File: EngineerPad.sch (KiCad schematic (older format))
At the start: 64 parts, among them J1 AVR ISP, J2 USB_A, SW1 SW_Push, SW10 SW_Push, SW11 SW_Push, SW12 SW_Push, SW13 SW_Push, SW14 SW_Push, SW15 SW_Push, SW16 SW_Push, SW17 SW_Push, SW18 SW_Push, SW19 SW_Push, SW2 SW_Push, SW20 SW_Push, SW21 SW_Push, SW22 SW_Push, SW23 SW_Push, SW3 SW_Push, SW4 SW_Push, SW5 SW_Push, SW6 SW_Push, SW7 SW_Push, SW8 SW_Push, SW9 SW_Push, U1 ATmega328P-PU, Y1 16MHz

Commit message: socket and low profile
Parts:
- SW21, SW22, SW23: footprint Button_Switch_Keyboard:SW_Cherry_MX_1.00u_PCB -> JSA:SW_PG1350
- U1: footprint Package_DIP:DIP-28_W7.62mm -> Package_DIP:DIP-28_W7.62mm_Socket
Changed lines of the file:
@@
 F 0 "U1" H 1206 3746 50  0000 R CNN
 F 1 "ATmega328P-PU" H 1206 3655 50  0000 R CNN
-F 2 "Package_DIP:DIP-28_W7.62mm" H 1850 3700 50  0001 C CIN
+F 2 "Package_DIP:DIP-28_W7.62mm_Socket" H 1850 3700 50  0001 C CIN
 F 3 "http://ww1.microchip.com/downloads/en/DeviceDoc/ATmega328_P%20AVR%20MCU%20with%20picoPower%20Technology%20Data%20Sheet%2040001984A.pdf" H 1850 3700 50  0001 C CNN
 	1    1850 3700
@@
 F 0 "SW23" H 10550 4685 50  0000 C CNN
 F 1 "SW_Push" H 10550 4594 50  0000 C CNN
-F 2 "Button_Switch_Keyboard:SW_Cherry_MX_1.00u_PCB" H 10550 4600 50  0001 C CNN
+F 2 "JSA:SW_PG1350" H 10550 4600 50  0001 C CNN
 F 3 "~" H 10550 4600 50  0001 C CNN
 	1    10550 4400
@@
 F 0 "SW22" H 10050 4685 50  0000 C CNN
 F 1 "SW_Push" H 10050 4594 50  0000 C CNN
-F 2 "Button_Switch_Keyboard:SW_Cherry_MX_1.00u_PCB" H 10050 4600 50  0001 C CNN
+F 2 "JSA:SW_PG1350" H 10050 4600 50  0001 C CNN
 F 3 "~" H 10050 4600 50  0001 C CNN
 	1    10050 4400
@@
 F 0 "SW21" H 9550 4685 50  0000 C CNN
 F 1 "SW_Push" H 9550 4594 50  0000 C CNN
-F 2 "Button_Switch_Keyboard:SW_Cherry_MX_1.00u_PCB" H 9550 4600 50  0001 C CNN
+F 2 "JSA:SW_PG1350" H 9550 4600 50  0001 C CNN
 F 3 "~" H 9550 4600 50  0001 C CNN
 	1    9550 4400

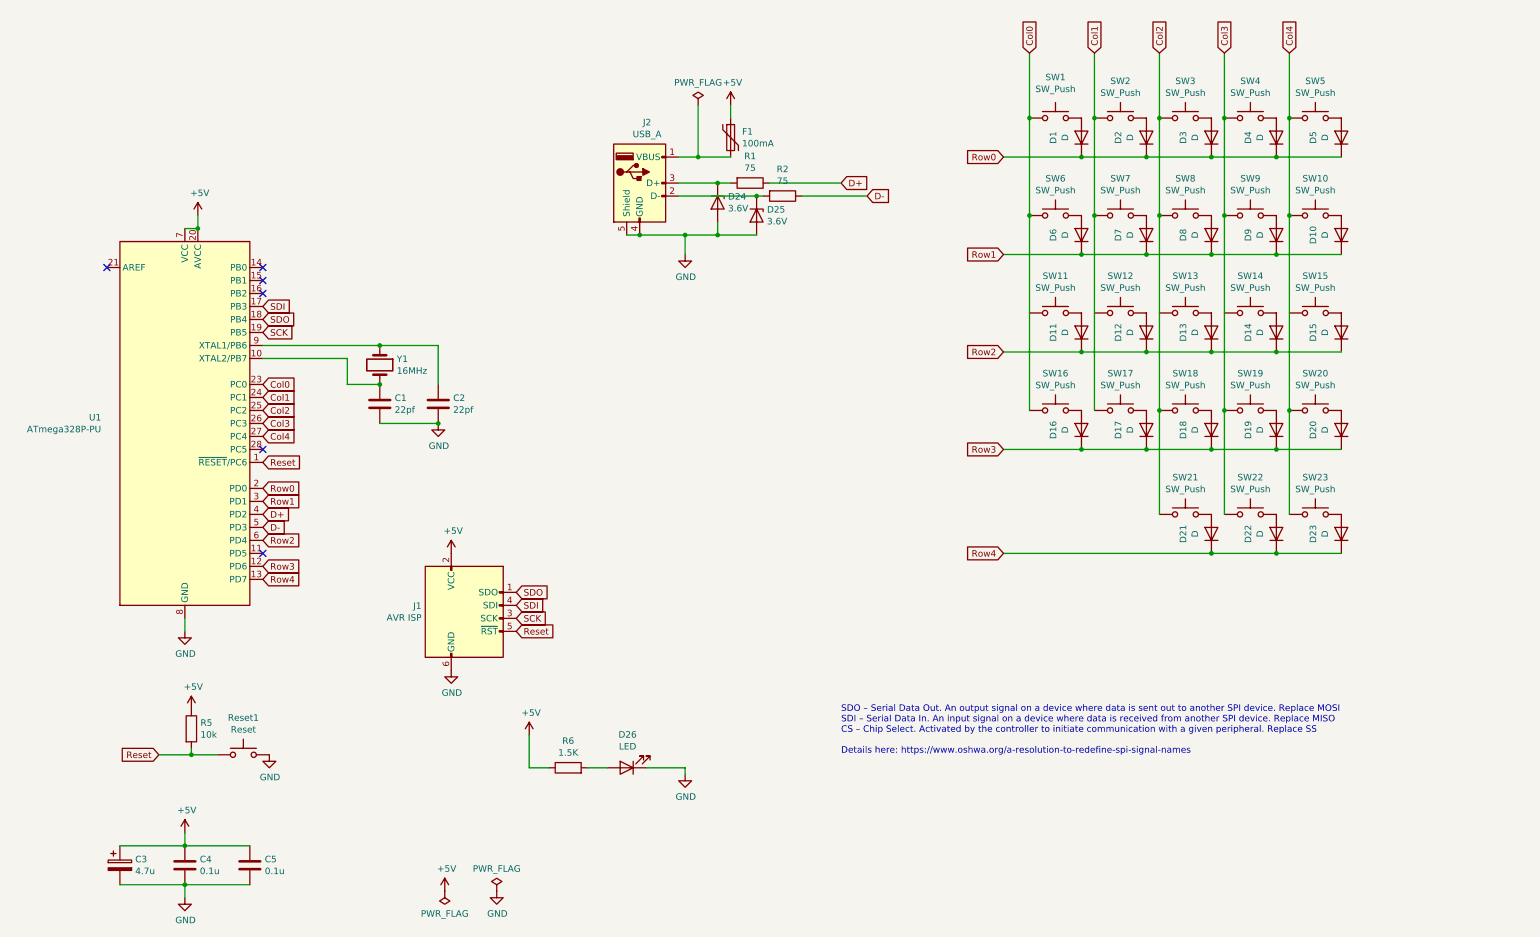
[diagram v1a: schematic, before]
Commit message: first layout
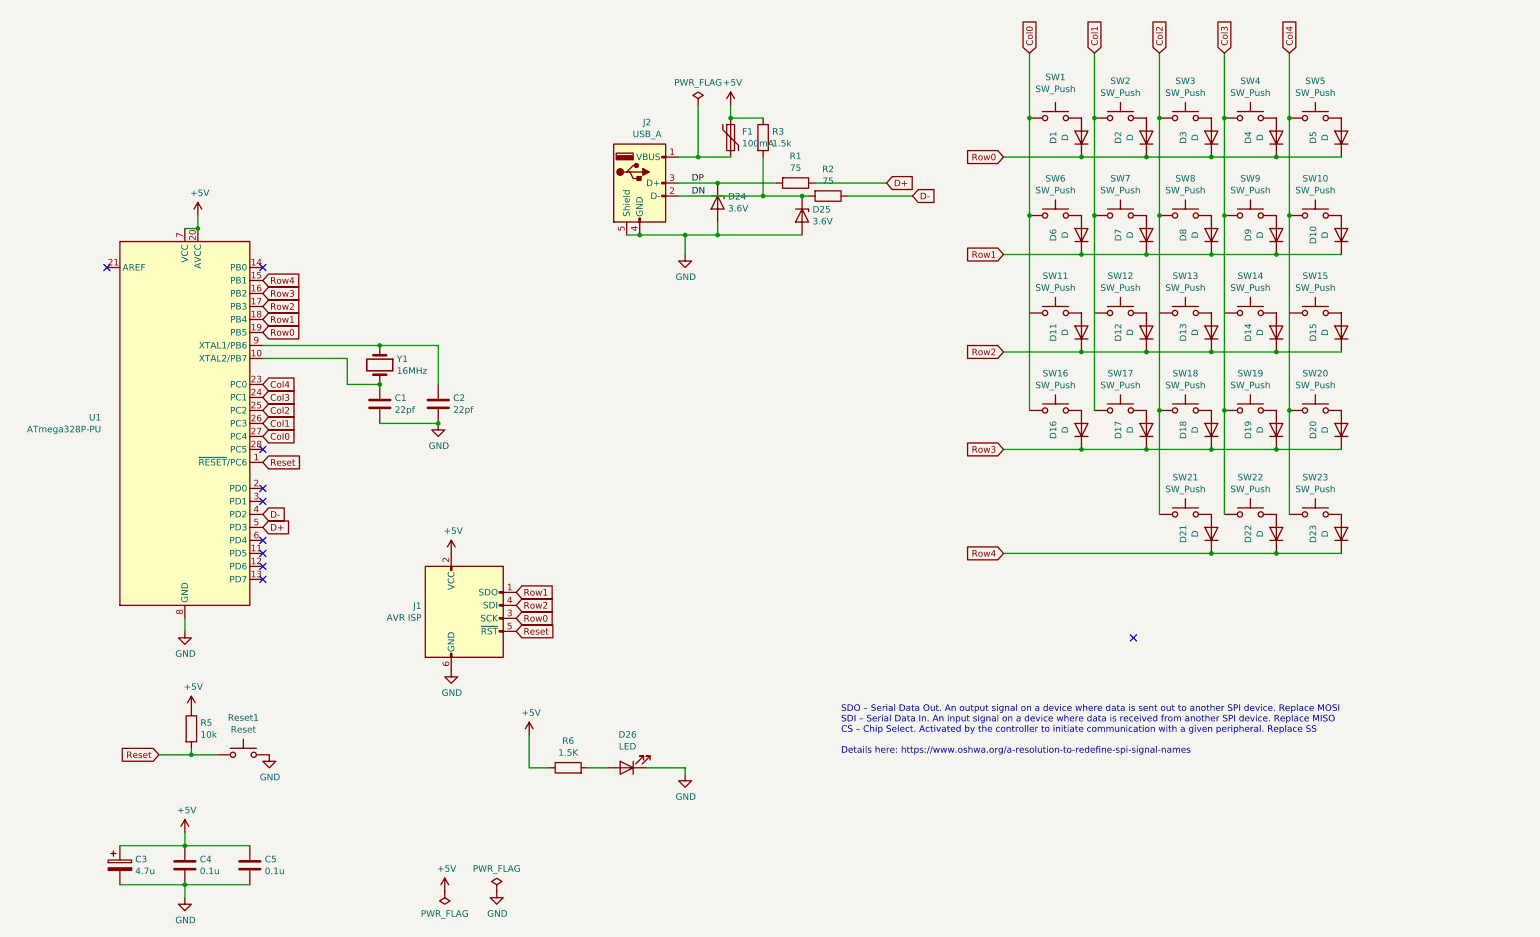
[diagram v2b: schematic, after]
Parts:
- added R3: 1.5k, Resistor_THT:R_Axial_DIN0204_L3.6mm_D1.6mm_P5.08mm_Horizontal, symbol Device:R
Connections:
- net SCK is gone; now on net Row0: J1.3 (SCK), U1.19 (PB5)
- net SDI is gone; now on net Row2: J1.4 (SDI), U1.17 (PB3)
- net SDO is gone; now on net Row1: J1.1 (SDO), U1.18 (PB4)
- net +5V: now also R3.1
- net Col0: now also U1.27 (PC4); no longer U1.23 (PC0)
- net Col1: now also U1.26 (PC3); no longer U1.24 (PC1)
- net Col3: now also U1.24 (PC1); no longer U1.26 (PC3)
- net Col4: now also U1.23 (PC0); no longer U1.27 (PC4)
- net D+: now also U1.5 (PD3); no longer U1.4 (PD2)
- net D-: now also U1.4 (PD2); no longer U1.5 (PD3)
- net Row0: no longer U1.2 (PD0)
- net Row1: no longer U1.3 (PD1)
- net Row2: no longer U1.6 (PD4)
- net Row3: now also U1.16 (PB2); no longer U1.12 (PD6)
- net Row4: now also U1.15 (PB1); no longer U1.13 (PD7)
- net DN: now reaches D25.1 (K), J2.2 (D-), R2.2
- net DN: now also R3.2
- net DP: now reaches D24.1 (K), J2.3 (D+), R1.2
- no-connect marks 6 -> 10
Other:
- moved on the sheet: D25, R1, R2
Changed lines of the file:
@@
 $EndComp
 Text GLabel 4400 5200 2    50   Input ~ 0
-SCK
+Row0
 Text GLabel 4400 5100 2    50   Input ~ 0
-SDI
-Text GLabel 4400 5000 2    50   Input ~ 0
-SDO
-Text GLabel 2450 3000 2    50   Input ~ 0
-SCK
-Text GLabel 2450 2900 2    50   Input ~ 0
-SDO
+Row2
+Text GLabel 2450 2700 2    50   Input ~ 0
+Row3
 Text GLabel 2450 2800 2    50   Input ~ 0
-SDI
+Row2
 $Comp
 L power:+5V #PWR09
@@
 Col0
 Connection ~ 8850 1350
-Text GLabel 2450 4200 2    50   Input ~ 0
+Text GLabel 2450 3000 2    50   Input ~ 0
 Row0
-Text GLabel 2450 4300 2    50   Input ~ 0
+Text GLabel 2450 2900 2    50   Input ~ 0
 Row1
-Text GLabel 2450 3400 2    50   Input ~ 0
+Text GLabel 2450 3800 2    50   Input ~ 0
 Col0
-Text GLabel 2450 3500 2    50   Input ~ 0
+Text GLabel 2450 3700 2    50   Input ~ 0
 Col1
 NoConn ~ 2450 2500
-NoConn ~ 2450 2600
-NoConn ~ 2450 2700
 NoConn ~ 1250 2500
+Text GLabel 2450 4500 2    50   Input ~ 0
+D+
 Text GLabel 2450 4400 2    50   Input ~ 0
-D+
-Text GLabel 2450 4500 2    50   Input ~ 0
 D-
 Text Notes 6900 6250 0    50   ~ 0
@@
 Text GLabel 10350 850  1    50   Input ~ 0
 Col4
-Text GLabel 2450 4600 2    50   Input ~ 0
-Row2
-Text GLabel 2450 4800 2    50   Input ~ 0
-Row3
-Text GLabel 2450 4900 2    50   Input ~ 0
+Text GLabel 2450 2600 2    50   Input ~ 0
 Row4
 Text GLabel 2450 3600 2    50   Input ~ 0
 Col2
-Text GLabel 2450 3700 2    50   Input ~ 0
+Text GLabel 2450 3500 2    50   Input ~ 0
 Col3
-Text GLabel 2450 3800 2    50   Input ~ 0
+Text GLabel 2450 3400 2    50   Input ~ 0
 Col4
 Connection ~ 8350 1350
@@
 L Device:R R1
 U 1 1 5F4818C7
-P 6200 1850
-F 0 "R1" V 5993 1850 50  0000 C CNN
-F 1 "75" V 6084 1850 50  0000 C CNN
-F 2 "Resistor_THT:R_Axial_DIN0204_L3.6mm_D1.6mm_P5.08mm_Horizontal" V 6130 1850 50  0001 C CNN
-F 3 "~" H 6200 1850 50  0001 C CNN
-	1    6200 1850
+P 6550 1850
+F 0 "R1" V 6343 1850 50  0000 C CNN
+F 1 "75" V 6434 1850 50  0000 C CNN
+F 2 "Resistor_THT:R_Axial_DIN0204_L3.6mm_D1.6mm_P5.08mm_Horizontal" V 6480 1850 50  0001 C CNN
+F 3 "~" H 6550 1850 50  0001 C CNN
+	1    6550 1850
 	0    1    1    0
 $EndComp
@@
 L Device:R R2
 U 1 1 5F48290F
-P 6450 1950
-F 0 "R2" V 6243 1950 50  0000 C CNN
-F 1 "75" V 6334 1950 50  0000 C CNN
-F 2 "Resistor_THT:R_Axial_DIN0204_L3.6mm_D1.6mm_P5.08mm_Horizontal" V 6380 1950 50  0001 C CNN
-F 3 "~" H 6450 1950 50  0001 C CNN
-	1    6450 1950
+P 6800 1950
+F 0 "R2" V 6593 1950 50  0000 C CNN
+F 1 "75" V 6684 1950 50  0000 C CNN
+F 2 "Resistor_THT:R_Axial_DIN0204_L3.6mm_D1.6mm_P5.08mm_Horizontal" V 6730 1950 50  0001 C CNN
+F 3 "~" H 6800 1950 50  0001 C CNN
+	1    6800 1950
 	0    1    1    0
 $EndComp
@@
 	5650 1850 5950 1850
 Wire Wire Line
-	5650 1950 6250 1950
-Wire Wire Line
-	6350 1850 6900 1850
-Text GLabel 6900 1850 2    50   Input ~ 0
+	6700 1850 7250 1850
+Text GLabel 7250 1850 2    50   Input ~ 0
 D+
-Text GLabel 7100 1950 2    50   Input ~ 0
+Text GLabel 7450 1950 2    50   Input ~ 0
 D-
 Wire Wire Line
-	6600 1950 7100 1950
+	6950 1950 7450 1950
 $Comp
 L Device:D_Zener D25
 U 1 1 5F49960F
-P 6250 2100
-F 0 "D25" V 6204 2180 50  0000 L CNN
-F 1 "3.6V" V 6295 2180 50  0000 L CNN
-F 2 "Diode_THT:D_DO-35_SOD27_P7.62mm_Horizontal" H 6250 2100 50  0001 C CNN
-F 3 "~" H 6250 2100 50  0001 C CNN
-	1    6250 2100
+P 6600 2100
+F 0 "D25" V 6554 2180 50  0000 L CNN
+F 1 "3.6V" V 6645 2180 50  0000 L CNN
+F 2 "Diode_THT:D_DO-35_SOD27_P7.62mm_Horizontal" H 6600 2100 50  0001 C CNN
+F 3 "~" H 6600 2100 50  0001 C CNN
+	1    6600 2100
 	0    1    1    0
 $EndComp
@@
 	5950 2150 5950 2250
 Connection ~ 5950 1850
-Wire Wire Line
-	5950 1850 6050 1850
-Connection ~ 6250 1950
-Wire Wire Line
-	6250 1950 6300 1950
+Connection ~ 6600 1950
+Wire Wire Line
+	6600 1950 6650 1950
 Wire Wire Line
 	5250 2250 5350 2250
@@
 Connection ~ 5350 2250
 Connection ~ 5950 2250
-Wire Wire Line
-	5950 2250 6250 2250
 Wire Wire Line
 	5700 2250 5700 2400
@@
 Wire Wire Line
 	5800 1250 5800 1650
+Wire Wire Line
+	5800 1650 6050 1650
+$Comp
+L Device:R R3
+U 1 1 5F481387
+P 6300 1500
+F 0 "R3" H 6370 1546 50  0000 L CNN
+F 1 "1.5k" H 6370 1455 50  0000 L CNN
+F 2 "Resistor_THT:R_Axial_DIN0204_L3.6mm_D1.6mm_P5.08mm_Horizontal" V 6230 1500 50  0001 C CNN
+F 3 "~" H 6300 1500 50  0001 C CNN
+	1    6300 1500
+	1    0    0    -1
+$EndComp
+Wire Wire Line
+	5650 1950 6300 1950
+Wire Wire Line
+	5950 1850 6400 1850
+Wire Wire Line
+	5950 2250 6600 2250
+Wire Wire Line
+	6300 1650 6300 1950
+Connection ~ 6300 1950
+Wire Wire Line
+	6300 1950 6600 1950
+Wire Wire Line
+	6300 1350 6050 1350
+Connection ~ 6050 1350
 Connection ~ 5800 1650
-Wire Wire Line
-	5800 1650 6050 1650
+Text Label 5750 1850 0    50   ~ 0
+DP
+Text Label 5750 1950 0    50   ~ 0
+DN
+NoConn ~ 2450 4900
+NoConn ~ 9150 5350
+Text GLabel 4400 5000 2    50   Input ~ 0
+Row1
+NoConn ~ 2450 4200
+NoConn ~ 2450 4300
+NoConn ~ 2450 4600
+NoConn ~ 2450 4800
 $EndSCHEMATC
